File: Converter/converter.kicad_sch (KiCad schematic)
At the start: 35 parts, among them IC1 NCP5109ADR2G, IC2 NCP5109ADR2G, J1 Conn_01x01, J2 Conn_01x01

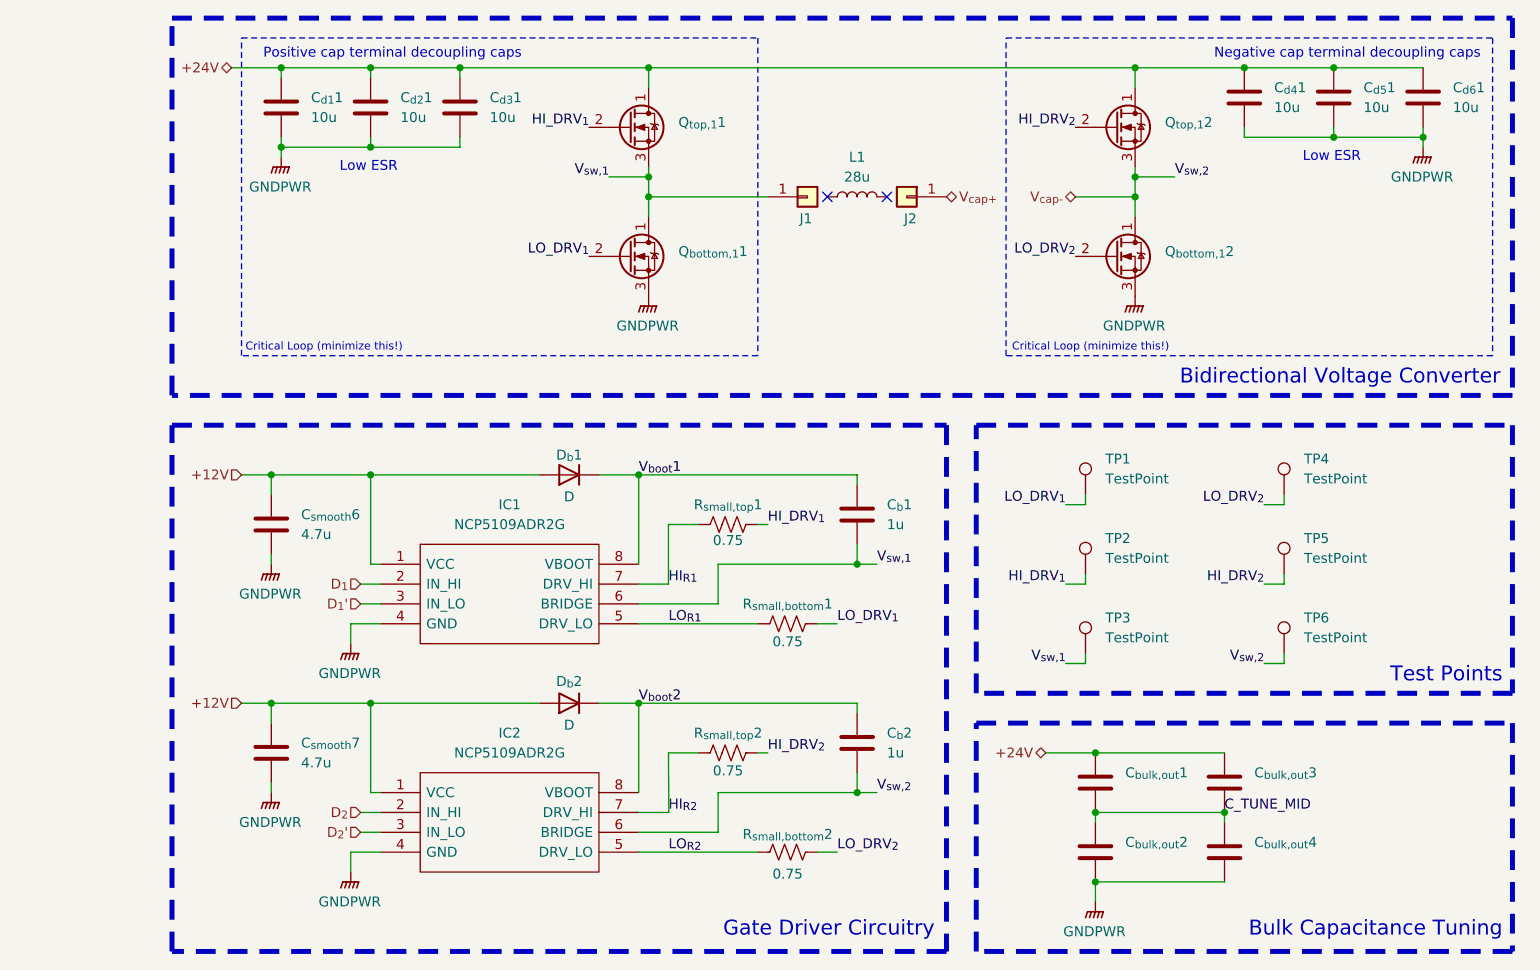
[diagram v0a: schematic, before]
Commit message: big progress on layout
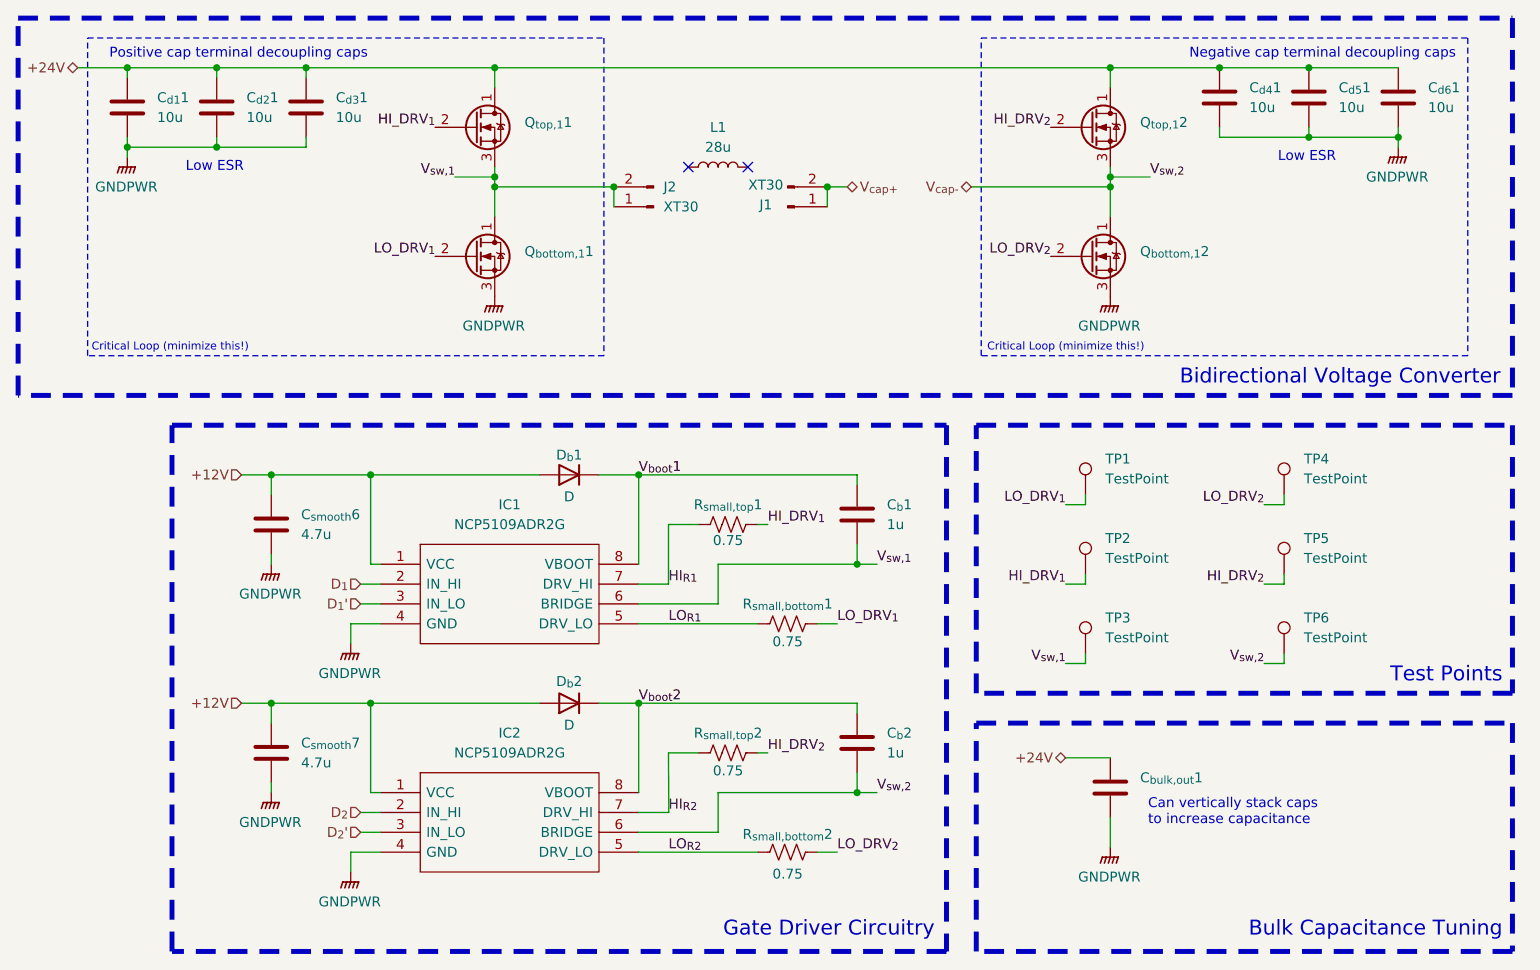
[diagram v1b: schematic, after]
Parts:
- removed C_{bulk,out}1, C_{bulk,out}3, C_{bulk,out}4: ~, Capacitor_SMD:C_0603_1608Metric_Pad1.08x0.95mm_HandSolder, symbol Device:C
- removed J1, J2: Conn_01x01, Robomaster_Passives:Inductor_wire_conn, symbol Connector_Generic:Conn_01x01
- added J1, J2: XT30, Connector_AMASS:AMASS_XT30UPB-F_1x02_P5.0mm_Vertical, symbol Connector:Conn_01x02_Pin
- C_{smooth}6, C_{smooth}7: footprint Capacitor_SMD:C_0805_2012Metric_Pad1.18x1.45mm_HandSolder -> Capacitor_SMD:C_0603_1608Metric_Pad1.08x0.95mm_HandSolder; Manufacturer_Part_Number 80-C0805X475J8RAUTO -> CL10A475KO8NNNC; Mouser Part Number 80-C0805X475J8RAUTO -> 187-CL10A475KO8NNNC
- renumbered C_{bulk,out}2 to C_{bulk,out}1
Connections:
- net C_TUNE_MID is gone; now on net +24V: C_{bulk,out}1.1
- net V_{cap+}: now also J1.1 (Pin_1), J1.2 (Pin_2)
- net V_{sw,1}: now also J2.1 (Pin_1), J2.2 (Pin_2)
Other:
- note added: "Can vertically stack caps to increase capacitance"
- moved on the sheet: C_{bulk,out}1, C_{d1}1, C_{d2}1, C_{d3}1, C_{d4}1, C_{d5}1, C_{d6}1, L1, Q_{bottom,1}1, Q_{bottom,1}2, Q_{top,1}1, Q_{top,1}2
